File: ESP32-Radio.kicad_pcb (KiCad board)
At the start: 2 copper layers, 119.8 x 71.5 mm, 72 parts, among them J1 Jack-DC, J11 Conn_01x04_Female, J2 BNC, J6 Audio_Jack, Q1 2N3904-SMD, Q2 2SC5706, Q3 2SC5706, T1 T50_SPLITTER, U1 LM358, U10 si5351, U11 LD33V, U2 LM358, U6 MCP1703A-2502_SOT223, U8 FST3253

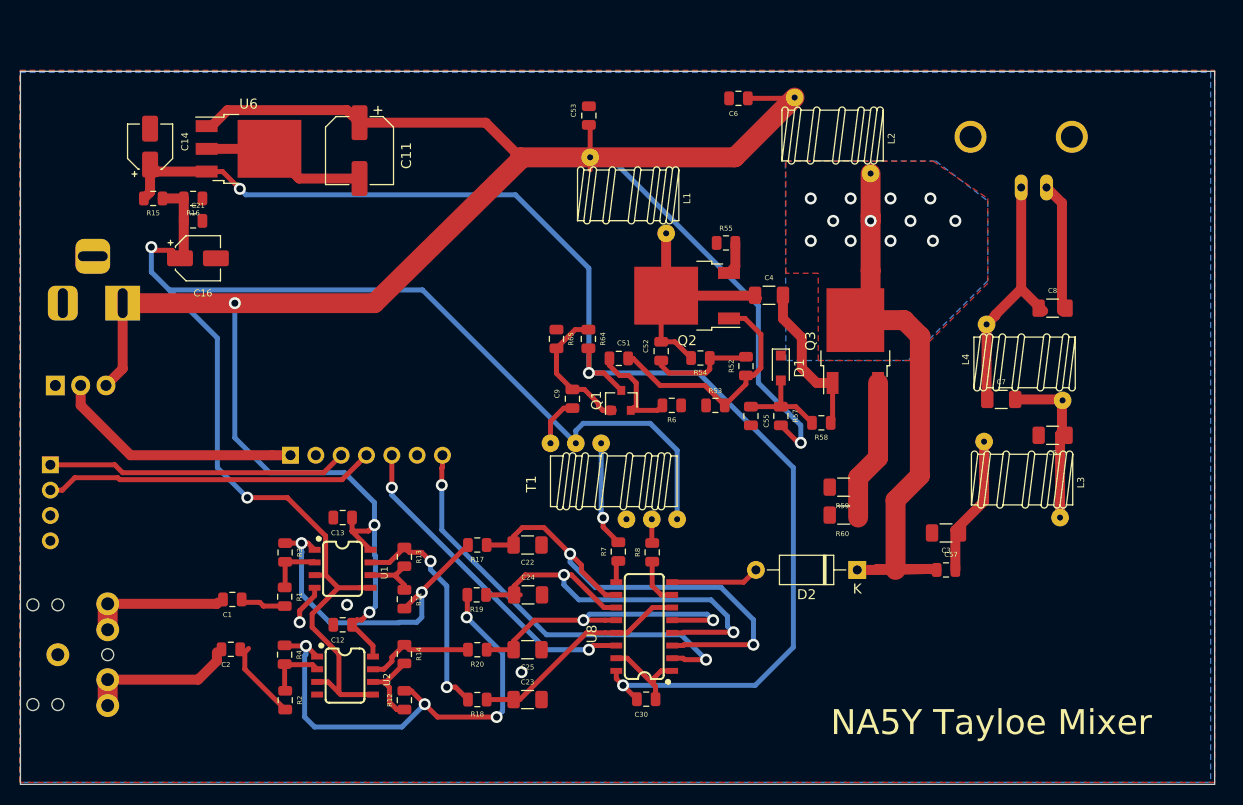
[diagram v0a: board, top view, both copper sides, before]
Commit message: created
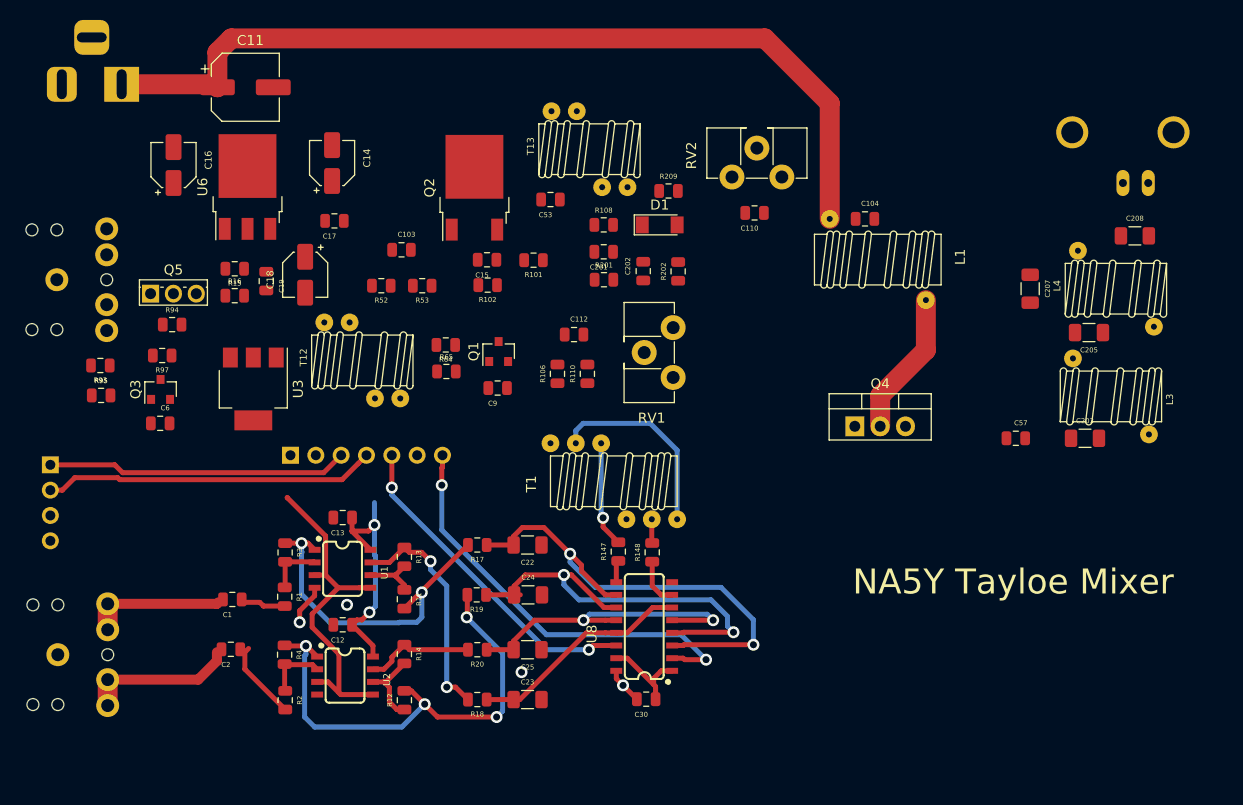
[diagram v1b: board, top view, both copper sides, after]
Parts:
- removed C21, C51, C52, C55: .1uF, Xenir:Capacitor 0805
- removed C4: 150pF, Xenir:Capacitor 1206
- removed C7: 33p, Xenir:Capacitor 1206
- removed D2: D_Zener, Diode_THT:D_A-405_P10.16mm_Horizontal
- removed L2: Inductor, Xenir:T37_Inductor
- removed R54: 10k, Xenir:Resistor 0805
- removed R55: 10, Xenir:Resistor 0805
- removed R57: 1k, Xenir:Resistor 0805
- removed R58: 100, Xenir:Resistor 0805
- removed R59, R60: 1, Xenir:Resistor 1206
- removed U11: LD33V, Package_TO_SOT_THT:TO-220-3_Vertical
- added C103: .1uF, Xenir:Capacitor 0805, F.Cu at (184.5, 107.9)
- added C104: .1uF, Xenir:Capacitor 0805, F.Cu at (230.9, 104.8)
- added C110: .1uF, Xenir:Capacitor 0805, F.Cu at (219.9, 109.2)
- added C112: .1uF, Xenir:Capacitor 0805, F.Cu at (201.8, 116.4)
- added C15: .1uF, Xenir:Capacitor 0805, F.Cu at (193.0, 113.9)
- added C17: .1uF, Xenir:Capacitor 0805, F.Cu at (177.7, 110.0)
- added C18: 22uF, Xenir:Cap_4x5.4, F.Cu at (175.3, 112.9)
- added C19: .1uF, Xenir:Capacitor 0805, F.Cu at (173.4, 113.5)
- added C201: .1uF, Xenir:Capacitor 0805, F.Cu at (204.7, 113.1)
- added C202: .1uF, Xenir:Capacitor 0805, F.Cu at (206.2, 112.5)
- added C207: 33p, Xenir:Capacitor 1206, F.Cu at (249.8, 114.3)
- added J4: Audio_Jack, Xenir:Audio_Jack, B.Cu at (151.9, 121.9)
- added Q4: IRF510, Package_TO_SOT_THT:TO-220-3_Vertical, F.Cu at (229.9, 128.1)
- added Q5: IRFU9024, Package_TO_SOT_THT:TO-251-3_Vertical, F.Cu at (159.3, 114.8)
- added R101: 18, Xenir:Resistor 0805, F.Cu at (197.7, 108.9)
- added R102: 18, Xenir:Resistor 0805, F.Cu at (193.1, 111.4)
- added R108: 100, Xenir:Resistor 0805, F.Cu at (204.7, 110.4)
- added R110: 62, Xenir:Resistor 0805, F.Cu at (205.6, 122.8)
- added R201: 33, Xenir:Resistor 0805, F.Cu at (204.8, 115.9)
- added R202: 10, Xenir:Resistor 0805, F.Cu at (214.7, 112.6)
- added R209: 2.7k, Xenir:Resistor 0805, F.Cu at (211.2, 107.0)
- added R93: 10k, Xenir:Resistor 0805, F.Cu at (154.3, 119.5)
- added R94: 10k, Xenir:Resistor 0805, F.Cu at (161.5, 120.4)
- added R95: 1.5k, Xenir:Resistor 0805, F.Cu at (154.3, 127.5)
- added R97: 10k, Xenir:Resistor 0805, F.Cu at (160.5, 118.5)
- added RV1: R_POT, Xenir:Trimpot Vertical, F.Cu at (210.3, 126.0)
- added RV2: R_POT, Xenir:Trimpot Vertical, F.Cu at (214.8, 101.7)
- added T12: T37-43 25T:8T, Xenir:T37 Transformer, F.Cu at (173.5, 121.5)
- added T13: T37-43 8T:4T, Xenir:T37 Transformer, F.Cu at (196.3, 100.3)
- added U3: AMS1117, Package_TO_SOT_SMD:SOT-223-3_TabPin2, F.Cu at (169.6, 124.3)
- C203: renamed from C3; value 220pF -> 150p
- C205: renamed from C5; value 470pF -> 330p
- C208: renamed from C8; value 330pF -> 150p
- D1: value 1N914 -> D_Zener; footprint Diode_SMD:D_SOD-323_HandSoldering -> Diode_SMD:D_MiniMELF
- L1: value Inductor -> T50-43 10T; footprint Xenir:T37_Inductor -> Xenir:T50_Inductor
- L3: value 10T T37-6 -> 14T T37-6
- L4: value 11T T37-6 -> 18T T37-6
- Q3: value 2SC5706 -> BS170F; footprint Package_TO_SOT_SMD:TO-252-2 -> Package_TO_SOT_SMD:SOT-23
- R106: renamed from R6; value 100 -> 62
- R52: value 1k -> 24k
- R53: value 1k -> 6.8k
- R64: value 4.7k -> 24k
- R65: value 4.7k -> 6.8k
- moved Q3 69.8 mm to (160.3, 124.4)
- moved C6 64.2 mm to (160.3, 125.3), turned to 0 degrees
- moved R52 40.5 mm to (182.4, 111.5), turned to 0 degrees
- moved R53 34.0 mm to (186.5, 111.5), turned to 0 degrees
- moved L1 27.5 mm to (241.0, 111.1)
- moved Q2 23.9 mm to (191.8, 104.2), turned to 90 degrees
- moved J1 22.0 mm to (156.4, 93.8)
- moved C11 21.5 mm to (168.7, 88.0), turned to 0 degrees
- moved C203 19.7 mm to (253.0, 127.0), turned to 0 degrees
- moved D1 18.8 mm to (210.3, 107.9), turned to 0 degrees
- moved C14 18.3 mm to (177.0, 101.7)
- moved R16 15.4 mm to (167.7, 117.5), turned to 180 degrees
- moved C57 14.9 mm to (246.1, 126.8)
- moved Q1 13.2 mm to (194.2, 120.6)
- moved L3 12.2 mm to (262.6, 125.1)
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- renumbered R7 to R147, R8 to R148
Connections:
- C16 pad 1: +2V5 -> 12V-On
- C53 pad 1: +12V -> 12V-On
- C6 pad 1: +12V -> Net-(C6-Pad1)
- D1 pad 1: GND -> Net-(C202-Pad2)
- L1 pad 2: Net-(C4-Pad1) -> Net-(C57-Pad1)
- Q1 pad 3: +5V -> Net-(Q1-Pad3)
- Q2 pad 2: Net-(C4-Pad1) -> Net-(Q2-Pad2)
- Q3 pad 1: Net-(C4-Pad2) -> Net-(C6-Pad1)
- Q3 pad 2: Net-(C57-Pad1) -> GND
- R52 pad 1: Net-(C52-Pad1) -> 12V-On
- R64 pad 1: +5V -> 12V-On
- T1 pad C1A: Net-(C9-Pad1) -> Net-(RV1-Pad1)
- U6 pad 1: +12V -> 12V-On
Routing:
- net +5V: track 133.7 -> 3.69 mm, vias 3 -> 1
- net +12V: track 224.2 -> 113.6 mm, vias 4 -> 2
- net +2V5: track 146.2 -> 54.2 mm, vias 2 -> 0
- net Net-(C57-Pad1): track 62.2 -> 14.6 mm, vias 12 -> 0
- net GND: track 51.8 -> 13.3 mm
- net Net-(C4-Pad1): track 33.2 -> 0.00 mm
- net Net-(C207-Pad1): track 25.8 -> 0.00 mm
- net +3V3: track 25.1 -> 0.00 mm
- net Net-(C103-Pad2): track 24.6 -> 0.00 mm
- net Net-(C205-Pad1): track 16.6 -> 0.00 mm
- net Net-(C4-Pad2): track 15.9 -> 0.00 mm
- net Net-(Q3-Pad3): track 14.3 -> 0.00 mm
- net Net-(C203-Pad1): track 14.1 -> 0.00 mm
- net Net-(C9-Pad2): track 14.0 -> 0.00 mm
- net Net-(C112-Pad1): track 10.7 -> 0.00 mm
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- removed copper zone on B.Cu, net GND
- removed copper zone on F.Cu, net GND
- removed copper zone on B.Cu, net Net-(C57-Pad1)
- removed copper zone on F.Cu, net Net-(C57-Pad1)
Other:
- board outline removed
